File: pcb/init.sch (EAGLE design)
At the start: 6 parts

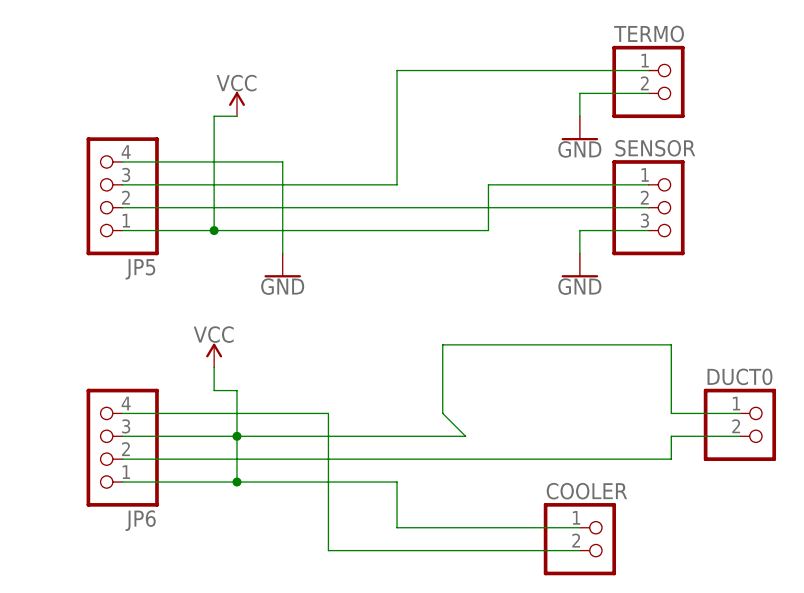
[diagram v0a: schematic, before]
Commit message: pcb
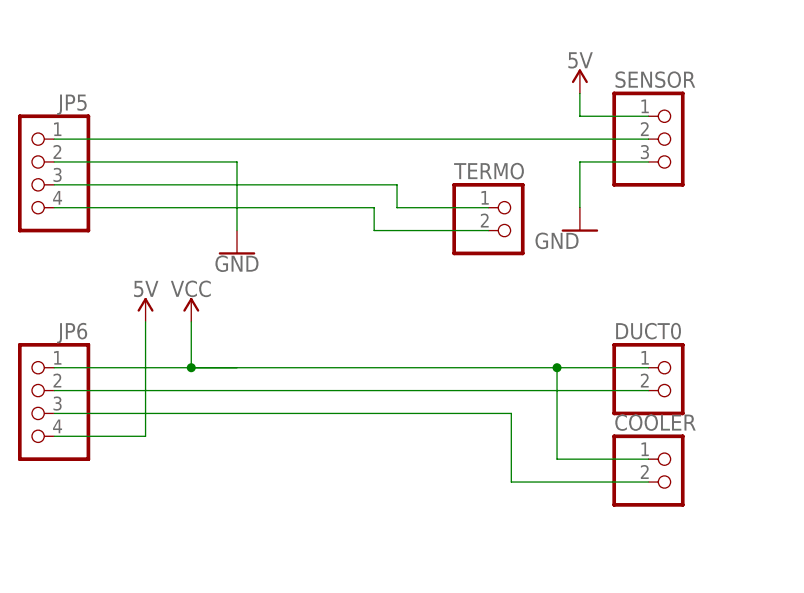
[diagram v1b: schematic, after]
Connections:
- removed net N$6: JP5.2, SENSOR.2
- new net 5V: JP6.4, SENSOR.1
- new net N$1: JP5.1, SENSOR.2
- new net N$2: COOLER.2, JP6.3
- net GND: now also JP5.2; no longer JP5.4, TERMO.2
- net N$5: now also JP5.4, TERMO.2; no longer COOLER.2, JP6.4
- net VCC: no longer JP5.1, JP6.3, SENSOR.1
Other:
- moved on the sheet: COOLER, DUCT0, JP5, JP6, SENSOR, TERMO
